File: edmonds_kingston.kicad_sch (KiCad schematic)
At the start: 15 parts

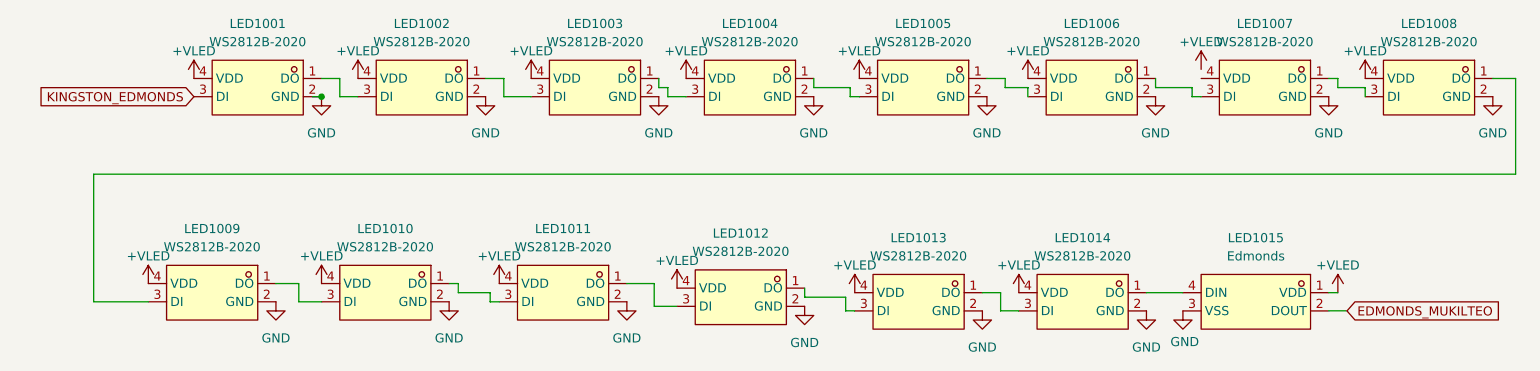
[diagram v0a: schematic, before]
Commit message: rev-b validation run
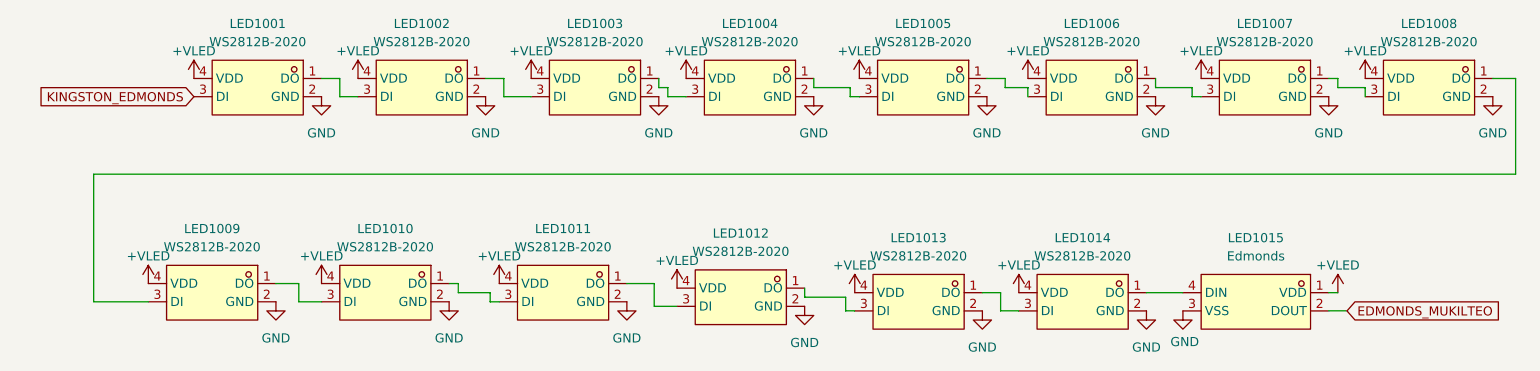
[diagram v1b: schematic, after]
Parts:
- LED1001, LED1002, LED1003, LED1004, LED1005, LED1006, LED1007, LED1008, LED1009, LED1010, LED1011, LED1012, LED1013, LED1014: LCSC Part C965555 -> C52917434
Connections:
- net +VLED: now also LED1007.4 (VDD)
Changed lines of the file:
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@@
 	(generator_version "10.0")
 	(paper "A4")
-	(junction
-		(at 65.405 44.45)
-		(diameter 0)
-		(color 0 0 0 0)
-	)
 	(wire
 		(pts
@@
 	(wire
 		(pts
-			(xy 65.405 44.45) (xy 64.135 44.45)
-		)
-		(stroke
-			(width 0)
-			(type default)
-		)
-	)
-	(wire
-		(pts
 			(xy 88.265 41.91) (xy 90.805 41.91)
 		)
@@
 	(symbol
 		(lib_id "power:VBUS")
-		(at 187.96 40.64 0)
+		(at 187.96 41.91 0)
 		(mirror y)
 		(unit 1)
@@
 		(dnp no)
 		(property "Reference" "#PWR0351"
-			(at 187.96 44.45 0)
+			(at 187.96 45.72 0)
 			(hide yes)
 			(show_name no)
@@
 		)
 		(property "Value" "+VLED"
-			(at 187.96 36.83 0)
+			(at 187.96 38.1 0)
 			(show_name no)
 			(do_not_autoplace no)
@@
 		)
 		(property "Footprint" ""
-			(at 187.96 40.64 0)
+			(at 187.96 41.91 0)
 			(hide yes)
 			(show_name no)
@@
 		)
 		(property "Datasheet" ""
-			(at 187.96 40.64 0)
+			(at 187.96 41.91 0)
 			(hide yes)
 			(show_name no)
@@
 		)
 		(property "Description" "Power symbol creates a global label with name \"VBUS\""
-			(at 187.96 40.64 0)
+			(at 187.96 41.91 0)
 			(hide yes)
 			(show_name no)
@@
 			)
 		)
-		(property "Datasheet" "https://lcsc.com/product-detail/Light-Emitting-Diodes-LED_Worldsemi-WS2812B-2020_C965555.html"
+		(property "Datasheet" "https://lcsc.com/product-detail/Light-Emitting-Diodes-LED_Worldsemi-WS2812B-2020_C52917434.html"
 			(at 180.34 84.455 0)
 			(hide yes)
@@
 			)
 		)
-		(property "LCSC Part" "C965555"
+		(property "LCSC Part" "C52917434"
 			(at 180.34 86.995 0)
 			(hide yes)
@@
 			)
 		)
-		(property "Datasheet" "https://lcsc.com/product-detail/Light-Emitting-Diodes-LED_Worldsemi-WS2812B-2020_C965555.html"
+		(property "Datasheet" "https://lcsc.com/product-detail/Light-Emitting-Diodes-LED_Worldsemi-WS2812B-2020_C52917434.html"
 			(at 181.61 54.61 0)
 			(hide yes)
@@
 			)
 		)
-		(property "LCSC Part" "C965555"
+		(property "LCSC Part" "C52917434"
 			(at 181.61 57.15 0)
 			(hide yes)
@@
 			)
 		)
-		(property "Datasheet" "https://lcsc.com/product-detail/Light-Emitting-Diodes-LED_Worldsemi-WS2812B-2020_C965555.html"
+		(property "Datasheet" "https://lcsc.com/product-detail/Light-Emitting-Diodes-LED_Worldsemi-WS2812B-2020_C52917434.html"
 			(at 158.115 54.61 0)
 			(hide yes)
@@
 			)
 		)
-		(property "LCSC Part" "C965555"
+		(property "LCSC Part" "C52917434"
 			(at 158.115 57.15 0)
 			(hide yes)
@@
 			)
 		)
-		(property "Datasheet" "https://lcsc.com/product-detail/Light-Emitting-Diodes-LED_Worldsemi-WS2812B-2020_C965555.html"
+		(property "Datasheet" "https://lcsc.com/product-detail/Light-Emitting-Diodes-LED_Worldsemi-WS2812B-2020_C52917434.html"
 			(at 112.395 54.61 0)
 			(hide yes)
@@
 			)
 		)
-		(property "LCSC Part" "C965555"
+		(property "LCSC Part" "C52917434"
 			(at 112.395 57.15 0)
 			(hide yes)
@@
 			)
 		)
-		(property "Datasheet" "https://lcsc.com/product-detail/Light-Emitting-Diodes-LED_Worldsemi-WS2812B-2020_C965555.html"
+		(property "Datasheet" "https://lcsc.com/product-detail/Light-Emitting-Diodes-LED_Worldsemi-WS2812B-2020_C52917434.html"
 			(at 205.74 54.61 0)
 			(hide yes)
@@
 			)
 		)
-		(property "LCSC Part" "C965555"
+		(property "LCSC Part" "C52917434"
 			(at 205.74 57.15 0)
 			(hide yes)
@@
 			)
 		)
-		(property "Datasheet" "https://lcsc.com/product-detail/Light-Emitting-Diodes-LED_Worldsemi-WS2812B-2020_C965555.html"
+		(property "Datasheet" "https://lcsc.com/product-detail/Light-Emitting-Diodes-LED_Worldsemi-WS2812B-2020_C52917434.html"
 			(at 65.405 54.61 0)
 			(hide yes)
@@
 			)
 		)
-		(property "LCSC Part" "C965555"
+		(property "LCSC Part" "C52917434"
 			(at 65.405 57.15 0)
 			(hide yes)
@@
 			)
 		)
-		(property "Datasheet" "https://lcsc.com/product-detail/Light-Emitting-Diodes-LED_Worldsemi-WS2812B-2020_C965555.html"
+		(property "Datasheet" "https://lcsc.com/product-detail/Light-Emitting-Diodes-LED_Worldsemi-WS2812B-2020_C52917434.html"
 			(at 133.985 54.61 0)
 			(hide yes)
@@
 			)
 		)
-		(property "LCSC Part" "C965555"
+		(property "LCSC Part" "C52917434"
 			(at 133.985 57.15 0)
 			(hide yes)
@@
 			)
 		)
-		(property "Datasheet" "https://lcsc.com/product-detail/Light-Emitting-Diodes-LED_Worldsemi-WS2812B-2020_C965555.html"
+		(property "Datasheet" "https://lcsc.com/product-detail/Light-Emitting-Diodes-LED_Worldsemi-WS2812B-2020_C52917434.html"
 			(at 228.6 54.61 0)
 			(hide yes)
@@
 			)
 		)
-		(property "LCSC Part" "C965555"
+		(property "LCSC Part" "C52917434"
 			(at 228.6 57.15 0)
 			(hide yes)
@@
 			)
 		)
-		(property "Datasheet" "https://lcsc.com/product-detail/Light-Emitting-Diodes-LED_Worldsemi-WS2812B-2020_C965555.html"
+		(property "Datasheet" "https://lcsc.com/product-detail/Light-Emitting-Diodes-LED_Worldsemi-WS2812B-2020_C52917434.html"
 			(at 157.48 84.455 0)
 			(hide yes)
@@
 			)
 		)
-		(property "LCSC Part" "C965555"
+		(property "LCSC Part" "C52917434"
 			(at 157.48 86.995 0)
 			(hide yes)
@@
 			)
 		)
-		(property "Datasheet" "https://lcsc.com/product-detail/Light-Emitting-Diodes-LED_Worldsemi-WS2812B-2020_C965555.html"
+		(property "Datasheet" "https://lcsc.com/product-detail/Light-Emitting-Diodes-LED_Worldsemi-WS2812B-2020_C52917434.html"
 			(at 88.265 54.61 0)
 			(hide yes)
@@
 			)
 		)
-		(property "LCSC Part" "C965555"
+		(property "LCSC Part" "C52917434"
 			(at 88.265 57.15 0)
 			(hide yes)
@@
 			)
 		)
-		(property "Datasheet" "https://lcsc.com/product-detail/Light-Emitting-Diodes-LED_Worldsemi-WS2812B-2020_C965555.html"
+		(property "Datasheet" "https://lcsc.com/product-detail/Light-Emitting-Diodes-LED_Worldsemi-WS2812B-2020_C52917434.html"
 			(at 107.95 83.185 0)
 			(hide yes)
@@
 			)
 		)
-		(property "LCSC Part" "C965555"
+		(property "LCSC Part" "C52917434"
 			(at 107.95 85.725 0)
 			(hide yes)
@@
 			)
 		)
-		(property "Datasheet" "https://lcsc.com/product-detail/Light-Emitting-Diodes-LED_Worldsemi-WS2812B-2020_C965555.html"
+		(property "Datasheet" "https://lcsc.com/product-detail/Light-Emitting-Diodes-LED_Worldsemi-WS2812B-2020_C52917434.html"
 			(at 83.185 83.185 0)
 			(hide yes)
@@
 			)
 		)
-		(property "LCSC Part" "C965555"
+		(property "LCSC Part" "C52917434"
 			(at 83.185 85.725 0)
 			(hide yes)
@@
 			)
 		)
-		(property "Datasheet" "https://lcsc.com/product-detail/Light-Emitting-Diodes-LED_Worldsemi-WS2812B-2020_C965555.html"
+		(property "Datasheet" "https://lcsc.com/product-detail/Light-Emitting-Diodes-LED_Worldsemi-WS2812B-2020_C52917434.html"
 			(at 59.055 83.185 0)
 			(hide yes)
@@
 			)
 		)
-		(property "LCSC Part" "C965555"
+		(property "LCSC Part" "C52917434"
 			(at 59.055 85.725 0)
 			(hide yes)
@@
 			)
 		)
-		(property "Datasheet" "https://lcsc.com/product-detail/Light-Emitting-Diodes-LED_Worldsemi-WS2812B-2020_C965555.html"
+		(property "Datasheet" "https://lcsc.com/product-detail/Light-Emitting-Diodes-LED_Worldsemi-WS2812B-2020_C52917434.html"
 			(at 132.715 83.82 0)
 			(hide yes)
@@
 			)
 		)
-		(property "LCSC Part" "C965555"
+		(property "LCSC Part" "C52917434"
 			(at 132.715 86.36 0)
 			(hide yes)
